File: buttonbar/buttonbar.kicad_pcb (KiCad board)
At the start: 2 copper layers, 65.9 x 54.7 mm, 44 parts, among them J1 Conn_01x08_Male, J2 Conn_01x06_Male, SW1 SW_Push, SW2 SW_Push, SW3 SW_Push, SW4 SW_Push, SW5 SW_Push, SW6 SW_Push, U1 74HC14D

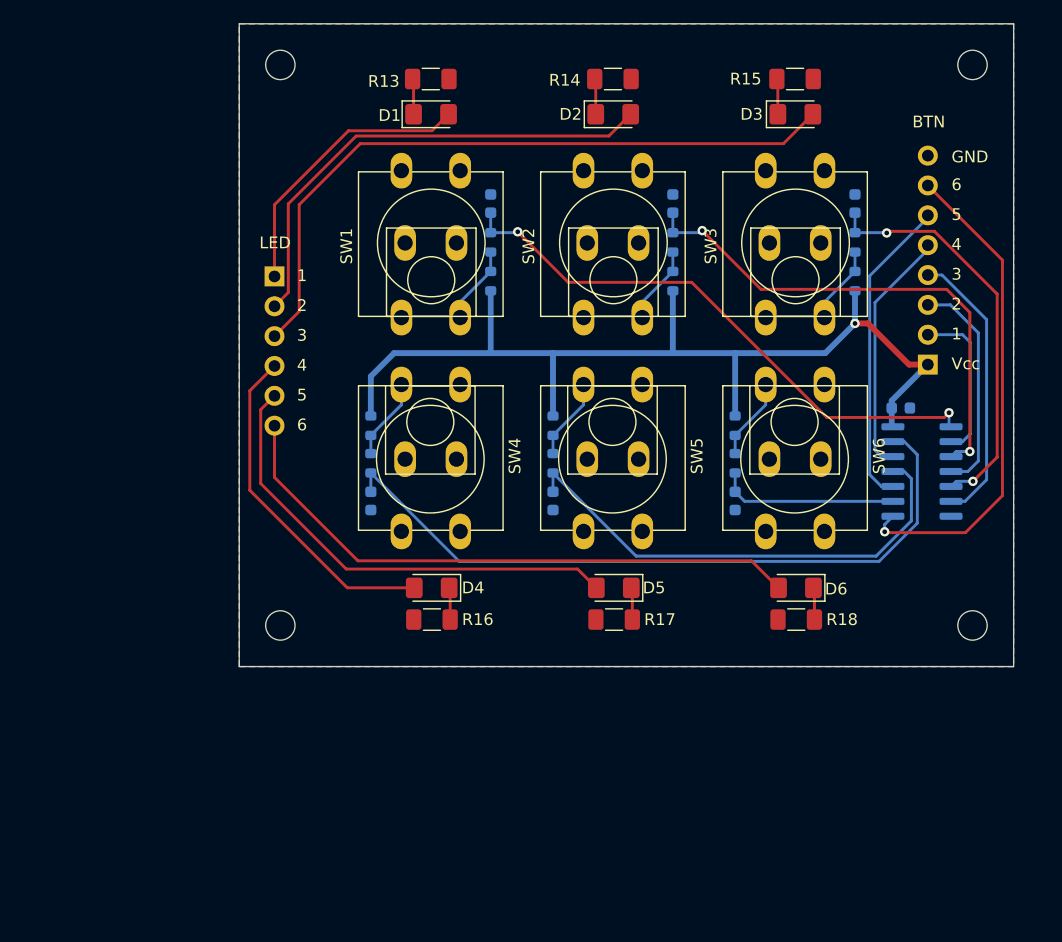
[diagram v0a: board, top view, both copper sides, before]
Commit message: Rev 2.1
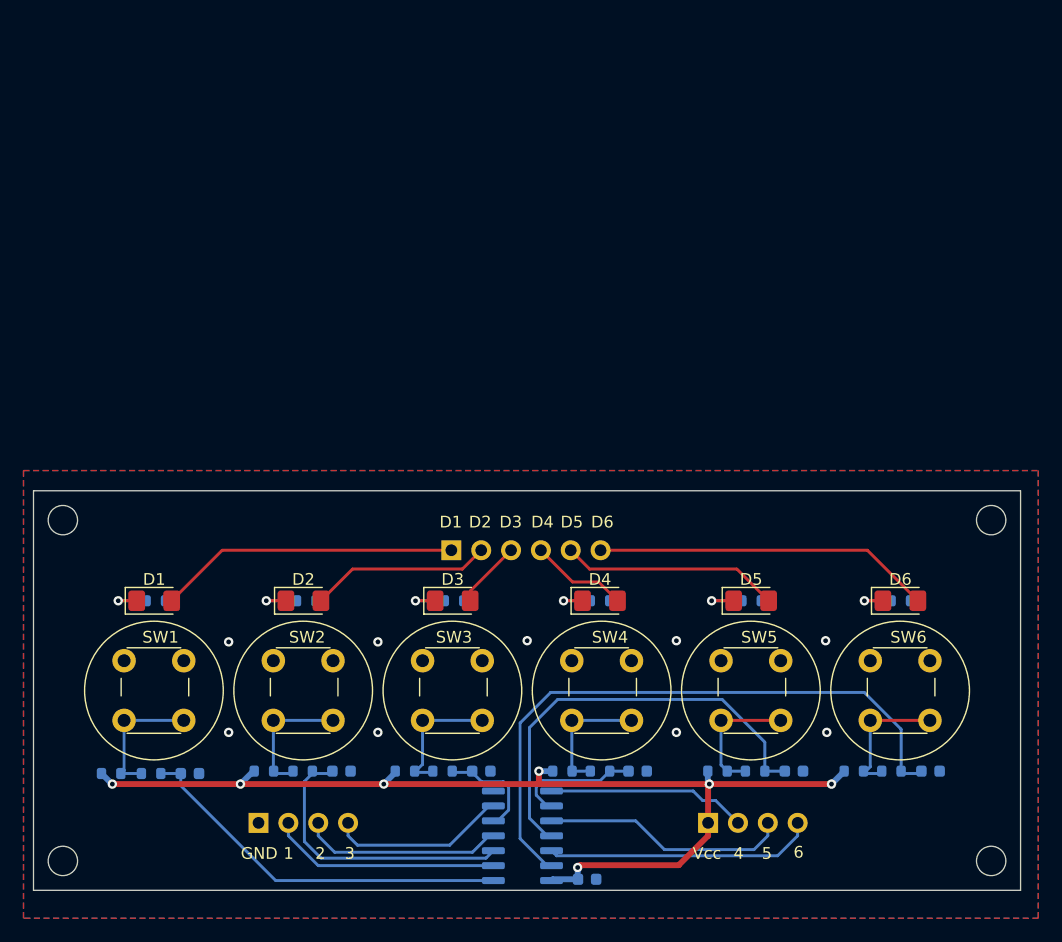
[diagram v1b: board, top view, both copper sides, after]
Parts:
- added J3: Conn_01x04_Male, Connector_PinHeader_2.54mm:PinHeader_1x04_P2.54mm_Vertical, B.Cu at (149.7, 113.8)
- J1: value Conn_01x08_Male -> Conn_01x04_Male; footprint Connector_PinHeader_2.54mm:PinHeader_1x08_P2.54mm_Vertical -> Connector_PinHeader_2.54mm:PinHeader_1x04_P2.54mm_Vertical
- R13, R14, R15, R16, R17, R18: value 680 1206 -> 680 0603; footprint Resistor_SMD:R_1206_3216Metric_Pad1.30x1.75mm_HandSolder -> Resistor_SMD:R_0603_1608Metric; moved to B.Cu
- SW1, SW2, SW3, SW4, SW5, SW6: footprint user:SW_PUSH-6.12mm -> user:SW_PUSH_5.08mm
- moved H4 80.0 mm to (94.8, 117.0)
- moved J1 69.0 mm to (111.4, 113.8), turned to -90 degrees
- moved H3 67.8 mm to (173.8, 117.0)
- moved H2 61.1 mm to (173.8, 88.0)
- moved C3 57.8 mm to (130.4, 109.4), turned to 0 degrees
- moved R6 57.1 mm to (127.1, 109.4), turned to 180 degrees
- moved R5 56.6 mm to (123.9, 109.4), turned to 0 degrees
- moved C2 55.9 mm to (118.5, 109.4), turned to 0 degrees
- moved R4 54.9 mm to (115.2, 109.4), turned to 180 degrees
- moved C1 54.8 mm to (105.6, 109.6), turned to 0 degrees
- moved R3 54.3 mm to (111.9, 109.4), turned to 0 degrees
- moved R2 53.6 mm to (102.3, 109.6), turned to 180 degrees
- moved R15 53.0 mm to (128.1, 94.9)
- moved R1 52.9 mm to (98.9, 109.6), turned to 0 degrees
- moved R14 51.5 mm to (115.5, 94.9)
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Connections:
- C6 pad 1: Net-(C6-Pad1) -> Net-(U1-Pad13)
- J1 pad 1: /Vcc -> GND
- R12 pad 1: Net-(C6-Pad1) -> Net-(U1-Pad13)
- U1 pad 12: /BTN_4 -> /BTN_6
- U1 pad 13: Net-(C4-Pad1) -> Net-(U1-Pad13)
- U1 pad 8: /BTN_6 -> /BTN_4
- U1 pad 9: Net-(C6-Pad1) -> Net-(C4-Pad1)
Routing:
- net Net-(U1-Pad13): track 0.00 -> 53.8 mm
- net Net-(D3-Pad2): track 58.9 -> 5.74 mm
- net Net-(C4-Pad1): track 60.9 -> 10.8 mm
- net Net-(D2-Pad2): track 41.5 -> 15.4 mm
- net Net-(C3-Pad1): track 34.9 -> 8.96 mm, vias 2 -> 0
- net Net-(D6-Pad2): track 51.2 -> 28.8 mm
- net Net-(D5-Pad2): track 40.2 -> 18.6 mm
- net Net-(D4-Pad2): track 28.9 -> 8.30 mm
- net /BTN_6: track 42.0 -> 22.9 mm, vias 1 -> 0
- net Net-(C2-Pad1): track 43.5 -> 24.7 mm, vias 2 -> 0
- net Net-(C1-Pad1): track 48.7 -> 32.7 mm, vias 2 -> 0
- net Net-(C6-Pad1): track 15.4 -> 0.00 mm
- net /BTN_3: track 24.0 -> 15.2 mm
- net /BTN_1: track 13.6 -> 19.6 mm
- net /Vcc: track 84.7 -> 90.6 mm, vias 1 -> 7
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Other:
- board size 65.9 x 54.7 mm -> 84 x 34 mm
- board text added: "D1"
- board text added: "D2"
- board text added: "D3"
- board text added: "D4"
- board text added: "D5"
- board text added: "D6"
- board text added: "https://github.com/bablokb/pcb-buttonbar Rev 2.1"
- board text removed: "BTN"
- board text removed: "LED"
- board text removed: "https://github.com/bablokb/pcb-buttonbar Rev 1.1"
